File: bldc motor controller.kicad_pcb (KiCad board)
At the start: 4 copper layers, 26 x 26 mm, 49 parts

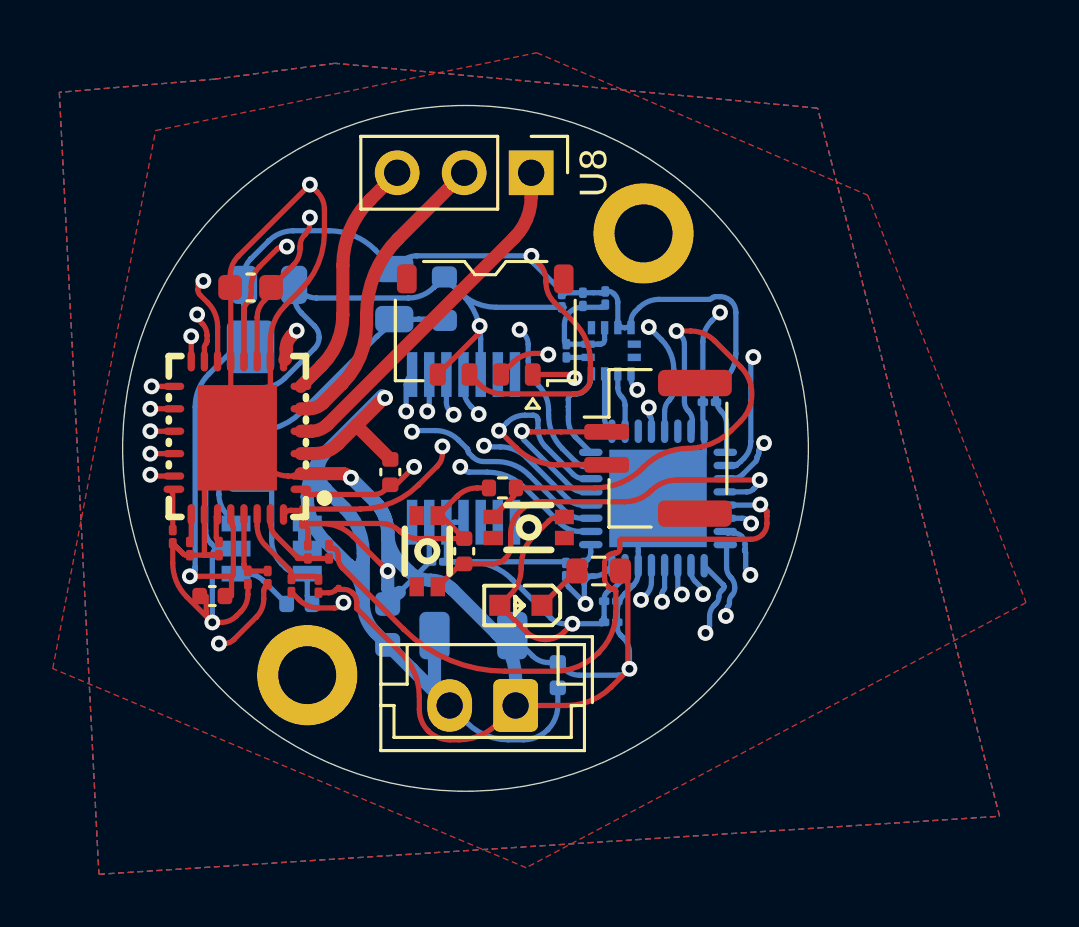
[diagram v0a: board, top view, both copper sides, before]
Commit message: 4 layer nice looking board
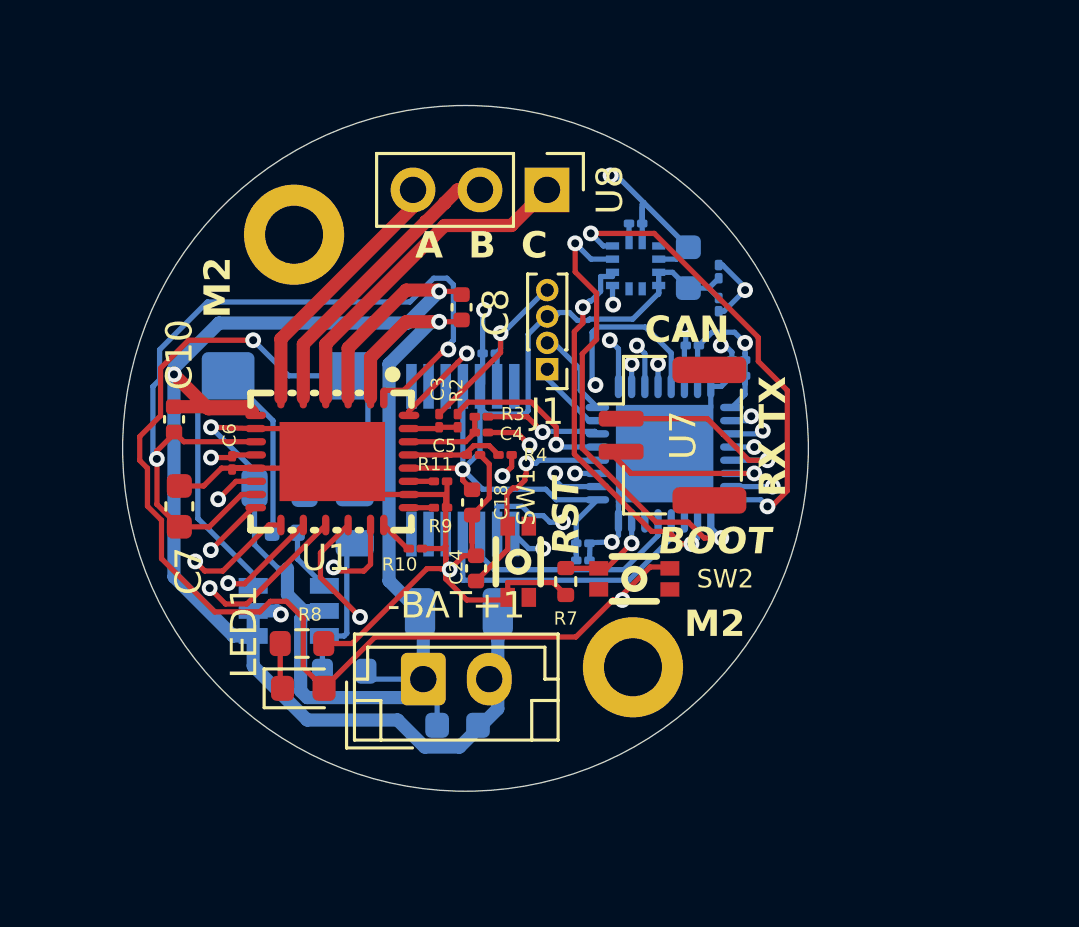
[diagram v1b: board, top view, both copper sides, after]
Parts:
- removed CN1: ~, Connector_JST:JST_EH_B2B-EH-A_1x02_P2.50mm_Vertical
- removed REF** (x2): MountingHole_2.2mm_M2_ISO14580_Pad, MountingHole:MountingHole_2.2mm_M2_ISO14580_Pad
- removed U2: ~, Connector_JST:JST_ACH_BM04B-ACHSS-A-GAN-ETF_1x04-1MP_P1.20mm_Vertical
- added -BAT+1: ~, Connector_JST:JST_EH_B2B-EH-A_1x02_P2.50mm_Vertical, F.Cu at (140.9, 96.8)
- added J1: Conn_01x04_Pin, Connector_PinHeader_1.00mm:PinHeader_1x04_P1.00mm_Vertical, F.Cu at (145.6, 85.0)
- added M2: MountingHole_2.2mm_M2_DIN965_Pad, MountingHole:MountingHole_2.2mm_M2_DIN965_Pad, F.Cu at (136.0, 79.9)
- added M2: MountingHole_2.2mm_M2_DIN965_Pad, MountingHole:MountingHole_2.2mm_M2_DIN965_Pad, F.Cu at (148.8, 96.3)
- added NT1: NetTie_2, NetTie:NetTie-2_SMD_Pad0.5mm, B.Cu at (135.8, 93.0)
- C22: footprint Capacitor_SMD:C_01005_0402Metric -> Capacitor_SMD:C_0603_1608Metric
- C8: moved to F.Cu
- LED1: footprint bldc-motor-footprints:LED0603-RD -> LED_SMD:LED_0603_1608Metric
- U1: value ~ -> C47023655
- U3: value ~ -> C529358
- U6: value ~ -> C126671
- moved R6 14.6 mm to (137.9, 96.5), turned to 0 degrees
- moved C8 14.4 mm to (142.3, 82.7), turned to -90 degrees
- moved R8 11.6 mm to (136.3, 95.4)
- moved C18 10.5 mm to (142.8, 90.0), turned to 90 degrees
- moved C12 10.3 mm to (151.1, 84.8), turned to 0 degrees
- moved C13 10.2 mm to (151.1, 84.1), turned to 0 degrees
- moved R4 10.1 mm to (144.0, 88.2), turned to 0 degrees
- moved C15 9.86 mm to (152.8, 84.7), turned to 0 degrees
- moved C14 9.84 mm to (152.8, 85.2), turned to 0 degrees
- moved C5 9.73 mm to (142.8, 88.2), turned to 0 degrees
- moved R3 9.63 mm to (143.1, 86.8), turned to 0 degrees
- moved R9 9.63 mm to (141.6, 90.2), turned to 0 degrees
- moved R10 9.21 mm to (140.6, 91.8), turned to 0 degrees
- moved LED1 8.83 mm to (136.3, 97.1), turned to 0 degrees
- moved R11 8.78 mm to (141.6, 89.2), turned to 0 degrees
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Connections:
- C1 pad 2: TI_AGND -> -BATT
- C8 pad 2: TI_AGND -> -BATT
- C9 pad 2: TI_AGND -> -BATT
- R6 pad 2: TI_AGND -> -BATT
- U1 pad 2: TI_AGND -> -BATT
- U4 pad 2: TI_AGND -> -BATT
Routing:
- net TI_AGND: track 153.6 -> 84.7 mm, vias 8 -> 9
- net -BATT: track 0.00 -> 48.4 mm, vias 0 -> 1
- net TI_VREF: track 96.4 -> 136.1 mm, vias 3 -> 5
- net +BATT: track 44.2 -> 77.4 mm, vias 2 -> 3
- net SOA: track 25.8 -> 6.56 mm
- net NSS1: track 33.3 -> 15.8 mm
- net SOB: track 20.8 -> 4.44 mm, vias 2 -> 1
- net BOOT0: track 19.8 -> 3.51 mm
- net TIM1_CH3N: track 30.9 -> 14.9 mm
- net ENAB_MAG: track 2.27 -> 17.2 mm, vias 0 -> 2
- net TI_FAULT: track 33.8 -> 19.4 mm
- net UART_RX: track 17.4 -> 3.06 mm, vias 2 -> 0
- net SDA1: track 3.75 -> 17.7 mm, vias 0 -> 2
- net ENAB_XL: track 2.24 -> 14.6 mm, vias 0 -> 2
- net TIM1_CH2N: track 23.1 -> 35.4 mm
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- removed copper zone on B.Cu, net TI_AGND
- removed copper zone on F.Cu, net TI_AGND
- removed copper zone on In2.Cu, net TI_AGND
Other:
- board text added: "A B C"
- board text added: "BOOT"
- board text added: "CAN"
- board text added: "RST"
- board text added: "RX TX"
